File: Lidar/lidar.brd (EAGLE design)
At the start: 29.2 x 35.2 mm, 5 parts, among them U1 ATTINY85-20P, X1 22-23-2051

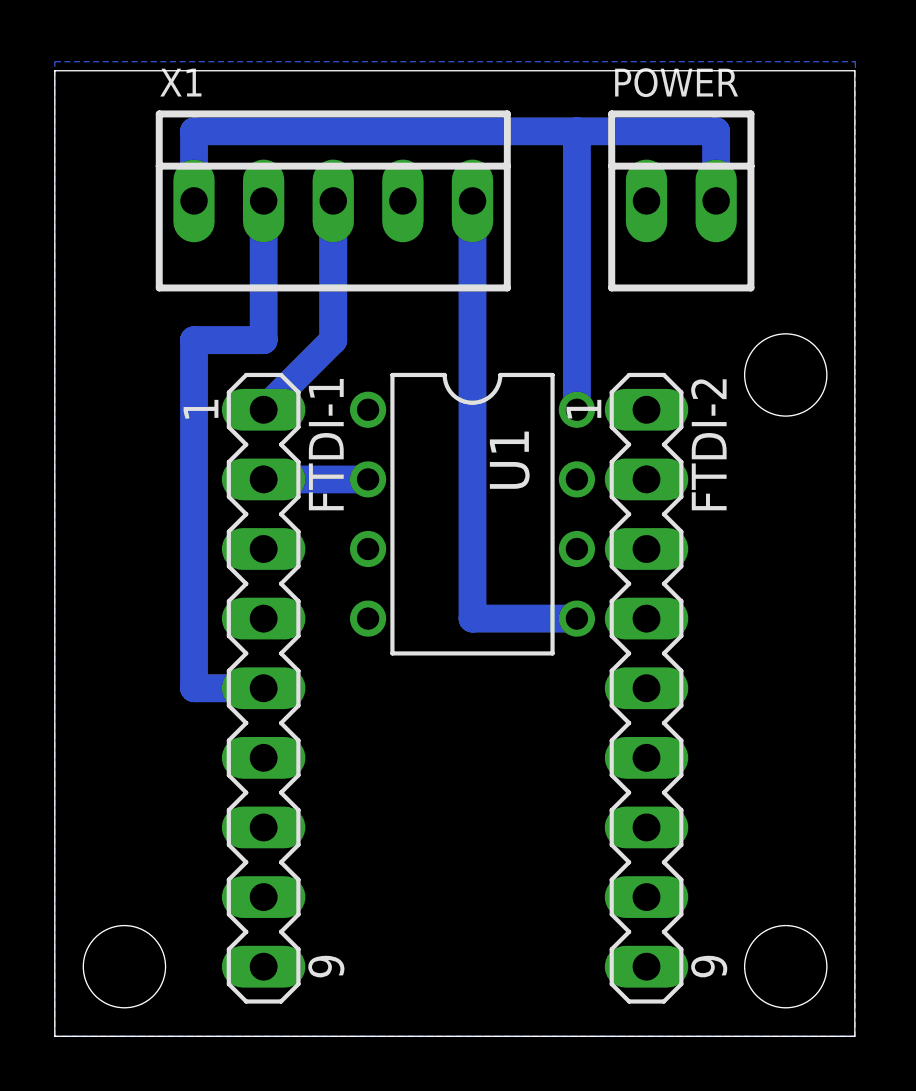
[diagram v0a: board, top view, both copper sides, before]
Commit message: fix board et gerber file
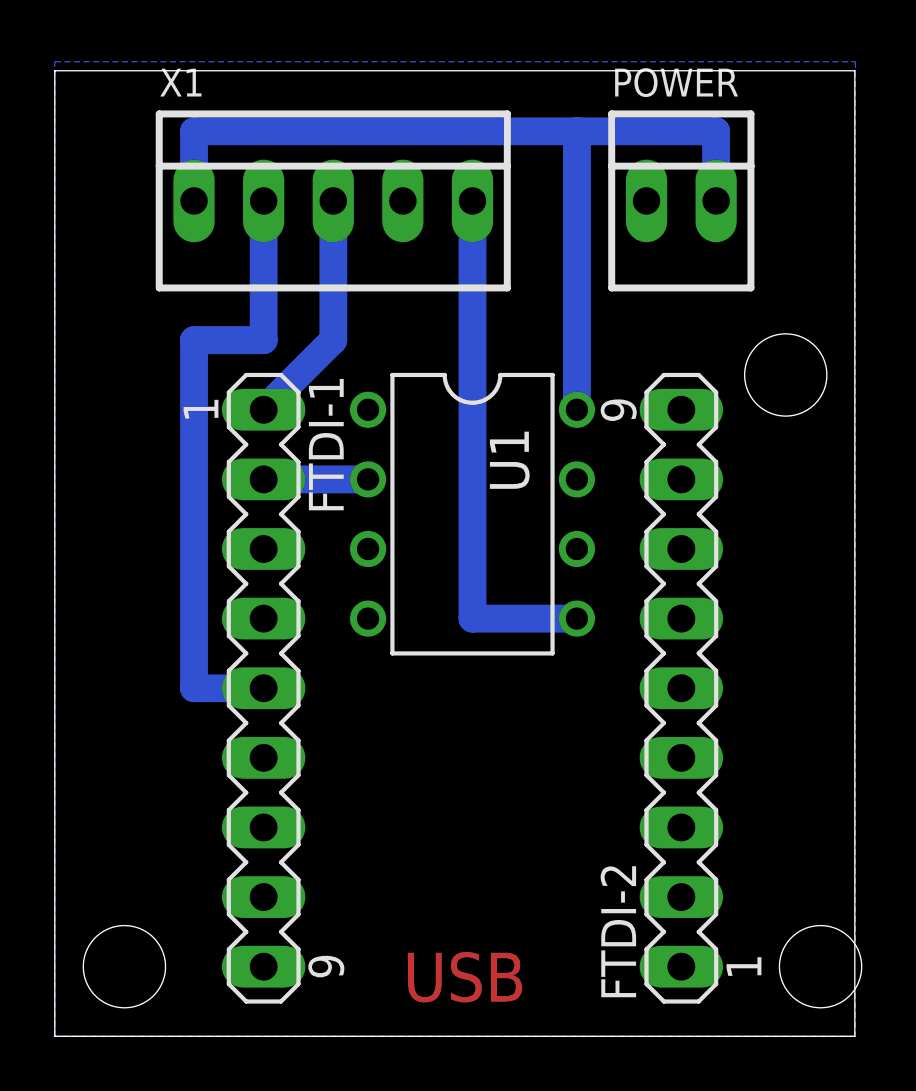
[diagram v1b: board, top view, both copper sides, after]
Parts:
- moved FTDI-2 1.27 mm to (22.9, 12.7), turned to 90 degrees
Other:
- board text added: "USB"
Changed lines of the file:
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@@
 <wire x1="0" y1="35.23" x2="0" y2="0" width="0" layer="20"/>
 <hole x="2.54" y="2.54" drill="3"/>
-<hole x="26.67" y="2.54" drill="3"/>
+<hole x="27.94" y="2.54" drill="3"/>
 <hole x="26.67" y="24.13" drill="3"/>
+<text x="12.7" y="1.27" size="1.778" layer="1">USB</text>
 </plain>
 <attributes>
@@
 <attribute name="VALUE" x="4.699" y="12.7" size="1.27" layer="27" ratio="10" rot="R270"/>
 </element>
-<element name="FTDI-2" library="con-lstb" library_urn="urn:adsk.eagle:library:162" package="MA09-1" package3d_urn="urn:adsk.eagle:package:8350/1" value="" x="21.59" y="12.7" smashed="yes" rot="R270">
-<attribute name="MF" value="" x="-1.27" y="-12.7" size="1.778" layer="27" rot="R270" display="off"/>
-<attribute name="MPN" value="" x="-1.27" y="-12.7" size="1.778" layer="27" rot="R270" display="off"/>
-<attribute name="NAME" x="23.241" y="24.13" size="1.27" layer="25" ratio="10" rot="R270"/>
-<attribute name="OC_FARNELL" value="unknown" x="-1.27" y="-12.7" size="1.778" layer="27" rot="R270" display="off"/>
-<attribute name="OC_NEWARK" value="unknown" x="-1.27" y="-12.7" size="1.778" layer="27" rot="R270" display="off"/>
-<attribute name="VALUE" x="18.669" y="12.7" size="1.27" layer="27" ratio="10" rot="R270"/>
+<element name="FTDI-2" library="con-lstb" library_urn="urn:adsk.eagle:library:162" package="MA09-1" package3d_urn="urn:adsk.eagle:package:8350/1" value="" x="22.86" y="12.7" smashed="yes" rot="R90">
+<attribute name="MF" value="" x="45.72" y="38.1" size="1.778" layer="27" rot="R90" display="off"/>
+<attribute name="MPN" value="" x="45.72" y="38.1" size="1.778" layer="27" rot="R90" display="off"/>
+<attribute name="NAME" x="21.209" y="1.27" size="1.27" layer="25" ratio="10" rot="R90"/>
+<attribute name="OC_FARNELL" value="unknown" x="45.72" y="38.1" size="1.778" layer="27" rot="R90" display="off"/>
+<attribute name="OC_NEWARK" value="unknown" x="45.72" y="38.1" size="1.778" layer="27" rot="R90" display="off"/>
+<attribute name="VALUE" x="25.781" y="12.7" size="1.27" layer="27" ratio="10" rot="R90"/>
 </element>
 <element name="U1" library="_hhn_attiny25_45_85" package="PDIP08_300MIL" value="ATTINY85-20P" x="15.24" y="19.05" smashed="yes" rot="R270">
